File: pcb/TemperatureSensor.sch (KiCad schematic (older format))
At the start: 1 part, among them U6 MCP9701T-E/TTCT-ND

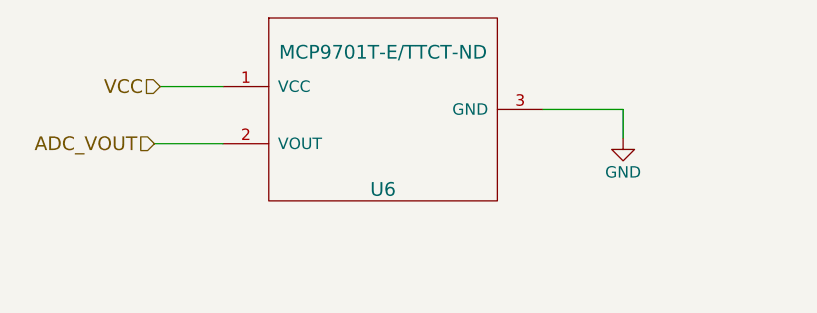
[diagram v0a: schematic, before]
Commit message: Clean up Kicad and TCC
Some changes in the
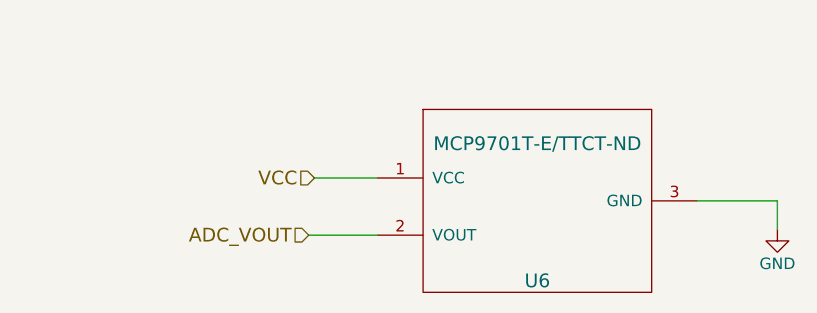
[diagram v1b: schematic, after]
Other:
- moved on the sheet: U6
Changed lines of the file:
@@
 $Descr A4 11693 8268
 encoding utf-8
-Sheet 6 10
-Title ""
+Sheet 10 10
+Title "Temperature Sensor Schematic"
 Date ""
-Rev ""
-Comp ""
+Rev "1"
+Comp "Universidade de Brasília - Campus Gama"
 Comment1 ""
 Comment2 ""
@@
 L pcb_v1-rescue:MCP9700T-E_LT U6
 U 1 1 5B5E76D9
-P 4225 3950
+P 4900 4350
 AR Path="/5B5E76D9" Ref="U6"  Part="1"
 AR Path="/5B5E7622/5B5E76D9" Ref="U6"  Part="1"
-F 0 "U6" H 5725 4450 60  0000 C CNN
-F 1 "MCP9701T-E/TTCT-ND" H 5725 5050 60  0000 C CNN
-F 2 "TO_SOT_Packages_SMD:SOT-23" H 5675 4700 60  0001 C CNN
-F 3 "https://www.digikey.com/product-detail/en/microchip-technology/MCP9701T-E-TT/MCP9701T-E-TTCT-ND/1987446" H 5675 4700 60  0001 C CNN
-	1    4225 3950
+F 0 "U6" H 6400 4850 60  0000 C CNN
+F 1 "MCP9701T-E/TTCT-ND" H 6400 5450 60  0000 C CNN
+F 2 "TO_SOT_Packages_SMD:SOT-23" H 6350 5100 60  0001 C CNN
+F 3 "https://www.digikey.com/product-detail/en/microchip-technology/MCP9701T-E-TT/MCP9701T-E-TTCT-ND/1987446" H 6350 5100 60  0001 C CNN
+	1    4900 4350
 	1    0    0    -1
 $EndComp
@@
 L power:GND #PWR010
 U 1 1 5B5E7776
-P 6775 3225
-F 0 "#PWR010" H 6775 2975 50  0001 C CNN
-F 1 "GND" H 6775 3075 50  0000 C CNN
-F 2 "" H 6775 3225 50  0001 C CNN
-F 3 "" H 6775 3225 50  0001 C CNN
-	1    6775 3225
+P 7450 3625
+F 0 "#PWR010" H 7450 3375 50  0001 C CNN
+F 1 "GND" H 7450 3475 50  0000 C CNN
+F 2 "" H 7450 3625 50  0001 C CNN
+F 3 "" H 7450 3625 50  0001 C CNN
+	1    7450 3625
 	1    0    0    -1
 $EndComp
 Wire Wire Line
-	6425 3100 6775 3100
+	7100 3500 7450 3500
 Wire Wire Line
-	6775 3100 6775 3225
-Text HLabel 4750 3000 0    60   Input ~ 0
+	7450 3500 7450 3625
+Text HLabel 5425 3400 0    60   Input ~ 0
 VCC
 Wire Wire Line
-	4750 3000 5025 3000
-Text HLabel 4725 3250 0    60   Input ~ 0
+	5425 3400 5700 3400
+Text HLabel 5400 3650 0    60   Input ~ 0
 ADC_VOUT
 Wire Wire Line
-	5025 3250 4725 3250
+	5700 3650 5400 3650
 $EndSCHEMATC
